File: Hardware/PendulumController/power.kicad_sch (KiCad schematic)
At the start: 8 parts, among them J301 19V Input, U301 NCV1117ST50T3G

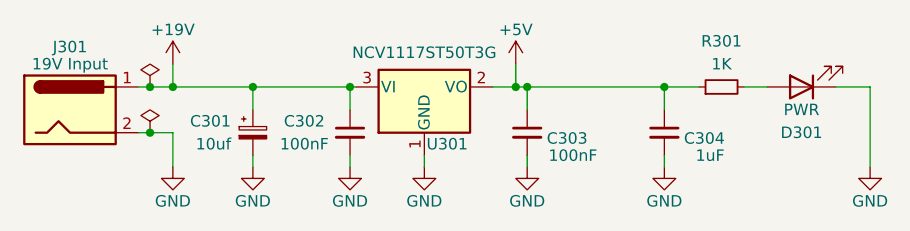
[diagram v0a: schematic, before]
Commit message: Cleanup readme and fix ERC
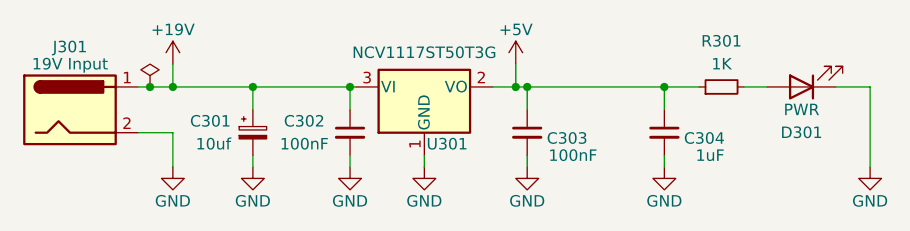
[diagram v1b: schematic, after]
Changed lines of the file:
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@@
   (junction (at 171.45 88.265) (diameter 0) (color 0 0 0 0)
   )
-  (junction (at 114.3 93.345) (diameter 0) (color 0 0 0 0)
-  )
   (junction (at 156.21 88.265) (diameter 0) (color 0 0 0 0)
   )
@@
     (stroke (width 0) (type default) (color 0 0 0 0))
   )
-  (wire (pts (xy 114.3 93.345) (xy 113.03 93.345))
-    (stroke (width 0) (type default) (color 0 0 0 0))
-  )
   (wire (pts (xy 180.34 88.265) (xy 182.88 88.265))
     (stroke (width 0) (type default) (color 0 0 0 0))
@@
     (stroke (width 0) (type default) (color 0 0 0 0))
   )
-  (wire (pts (xy 116.84 93.345) (xy 114.3 93.345))
+  (wire (pts (xy 113.03 93.345) (xy 116.84 93.345))
     (stroke (width 0) (type default) (color 0 0 0 0))
   )
@@
       (effects (font (size 1.27 1.27)) hide)
     )
-    (pin "1")
-  )
-  (symbol (lib_id "power:PWR_FLAG") (at 114.3 93.345 0) (unit 1)
-    (in_bom yes) (on_board yes) (fields_autoplaced)
-    (property "Reference" "#FLG?" (id 0) (at 114.3 91.44 0)
-      (effects (font (size 1.27 1.27)) hide)
-    )
-    (property "Value" "PWR_FLAG" (id 1) (at 114.3 87.63 0)
-      (effects (font (size 1.27 1.27)) hide)
-    )
-    (property "Footprint" "" (id 2) (at 114.3 93.345 0)
-      (effects (font (size 1.27 1.27)) hide)
-    )
-    (property "Datasheet" "~" (id 3) (at 114.3 93.345 0)
-      (effects (font (size 1.27 1.27)) hide)
-    )
